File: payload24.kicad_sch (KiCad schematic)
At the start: 21 parts, among them J1 532540370, J2 532540370, J3 460150206, J4 532540370, Q1 CSD19503KCS, Q2 CSD19503KCS, SW1 FingerTech

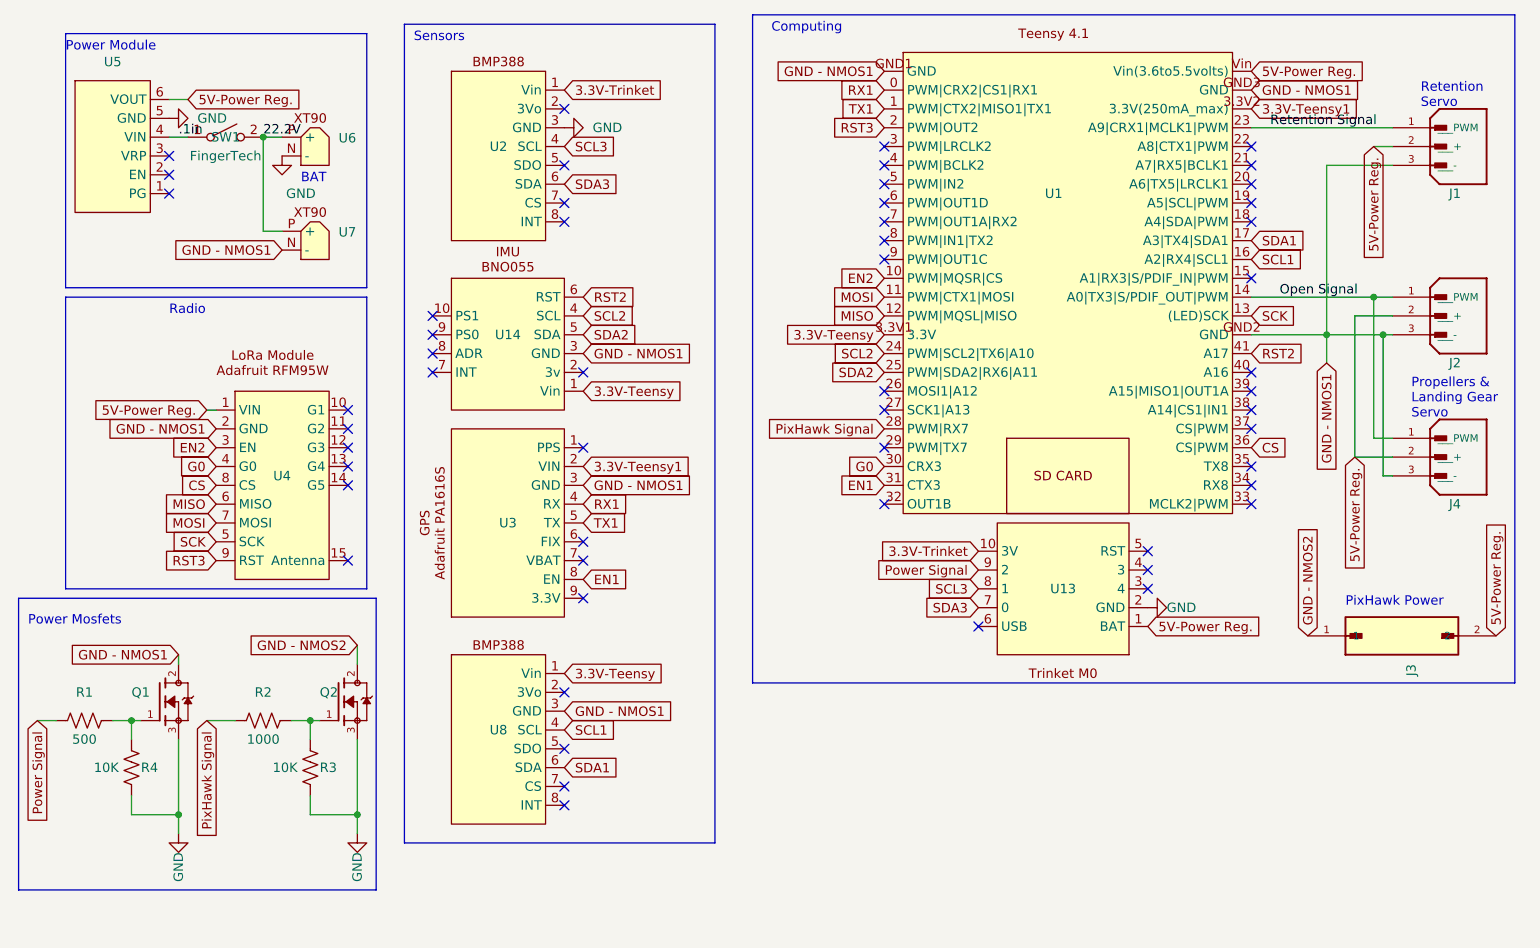
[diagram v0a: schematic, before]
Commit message: PCB laid out
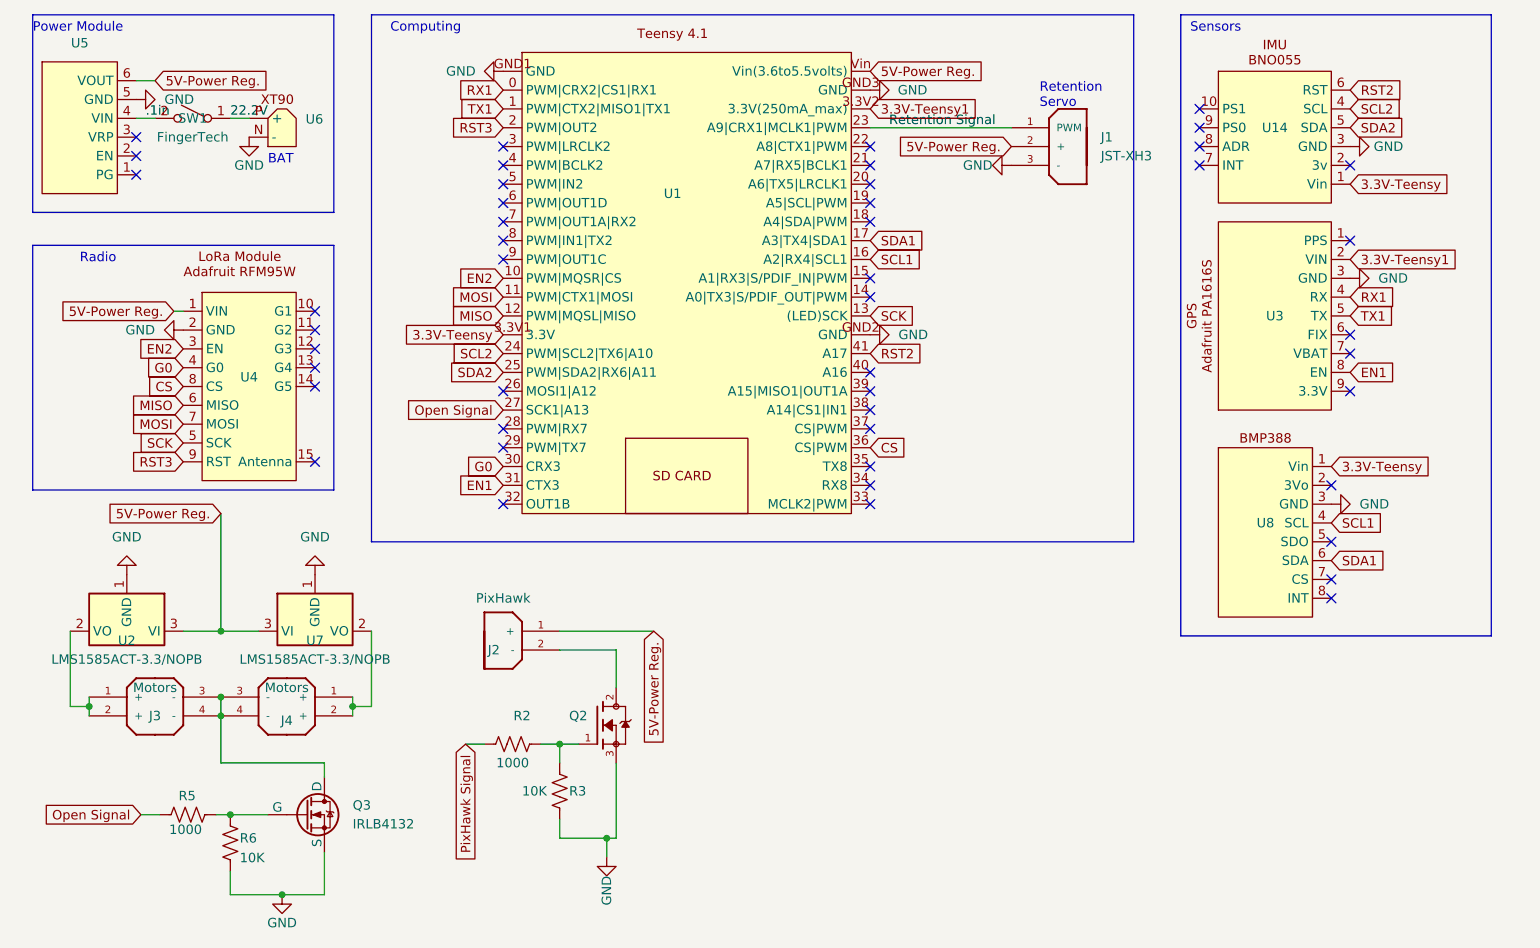
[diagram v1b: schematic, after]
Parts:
- removed J1, J2, J4: 532540370, JST-XH3:JST-XH3, symbol molexConnector:532540370
- removed J3: 460150206, JST-XH2:JST-XH2, symbol molex2pin:460150206
- removed Q1: CSD19503KCS, teensyMosfet:teensyMosfet, symbol teensyMosfet:CSD19503KCS
- removed R1: 500, 500Ohm:RESC3216X65N, symbol Device:R_US
- removed R4: 10K, 10KOhm:RESC3216X70N, symbol Device:R_US
- removed U13: ~, Trinket M0:Trinket M0, symbol Trinket M0:Trinket_M0
- removed U2: ~, BMP388:BMP388, symbol BMP388:BMP388
- removed U7: ~, XT60:AMASS_XT60-M, symbol PowerConnectors:XT90
- added J1: JST-XH3, JST-XH3:JST-XH3, symbol 532540370:JST-XH3
- added J2: PixHawk, JST-XH2:JST-XH2, symbol 532540370:JST-XH2
- added J3, J4: Motors, JST-XH3:JST-XH4, symbol 532540370:JST-XH4
- added Q3: IRLB4132, teensyMosfet:teensyMosfet, symbol Simulation_SPICE:NMOS
- added R5: 1000, 1kOhm:RESC3216X70N, symbol Device:R_US
- added R6: 10K, 10KOhm:RESC3216X70N, symbol Device:R_US
- added U2, U7: LMS1585ACT-3.3/NOPB, teensyMosfet:vRegulator, symbol Regulator_Linear:LD1117S33TR_SOT223
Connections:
- net GND - NMOS1 is gone; now on net GND: U1.GND1 (GND), U1.GND2 (GND), U1.GND3 (GND), U14.3 (GND), U3.3 (GND), U4.2 (GND), U8.3 (GND)
- net .1in: now also SW1.2 (B); no longer SW1.1 (A)
- net 22.2V: now also SW1.1 (A); no longer SW1.2 (B)
- net 5V-Power Reg.: now also J1.2 (+), J2.1 (+), U2.3 (VI), U7.3 (VI)
- net GND: now also J1.3 (-), Q3.3 (S), R6.2, U2.1 (GND), U7.1 (GND)
- net Open Signal: now also U1.27 (SCK1|A13), R5.1; no longer U1.14 (A0|TX3|S/PDIF_OUT|PWM)
- net PixHawk Signal: no longer U1.28 (PWM|RX7)
- net Retention  Signal: now also J1.1 (PWM)
- net GND - NMOS2: no longer names the net of Q2.2
- net GND - NMOS2: now also J2.2 (-)
- new net: J3.3 (-), J3.4 (-), J4.3 (-), J4.4 (-), Q3.1 (D)
- new net: Q3.2 (G), R5.2, R6.1
- new net: J4.1 (+), J4.2 (+), U7.2 (VO)
- new net: J3.1 (+), J3.2 (+), U2.2 (VO)
- no-connect marks 54 -> 47
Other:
- note removed: "PixHawk Power"
- note removed: "Power Mosfets"
- note removed: "Propellers & Landing Gear Servo"
- company: Anthony Konstantinidi and Kathleen Arrington -> (none)
- moved on the sheet: SW1, U1, U14, U3, U4, U5, U6, U8
